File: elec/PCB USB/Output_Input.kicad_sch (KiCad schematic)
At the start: 8 parts, among them J501 Conn_I2C_Écran, SW501 RotaryEncoder_Switch

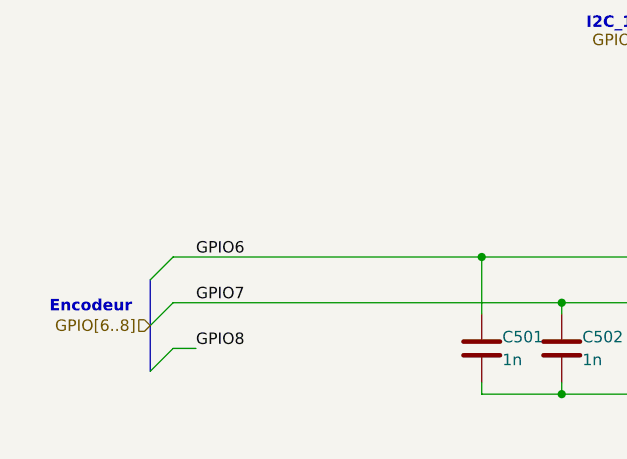
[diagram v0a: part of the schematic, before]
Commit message: push???
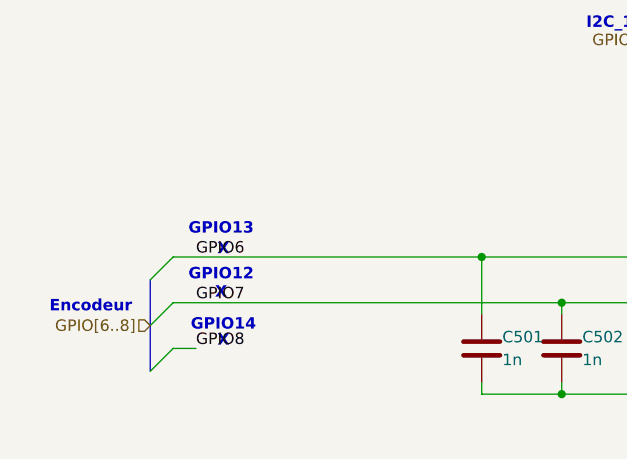
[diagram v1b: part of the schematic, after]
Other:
- note added: "GPIO12"
- note added: "GPIO13"
- note added: "GPIO14"
- note added: "X"
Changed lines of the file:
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@@
+		)
+	)
+	(text "X"
+		(exclude_from_sim no)
+		(at 94.488 84.328 0)
+		(effects
+			(font
+				(size 1.27 1.27)
+				(thickness 0.254)
+				(bold yes)
+				(color 255 24 7 1)
+			)
+		)
+	)
+	(text "GPIO13"
+		(exclude_from_sim no)
+		(at 94.234 71.882 0)
+		(effects
+			(font
+				(size 1.27 1.27)
+				(thickness 0.254)
+				(bold yes)
+				(color 34 86 25 1)
+			)
+		)
+	)
+	(text "X"
+		(exclude_from_sim no)
+		(at 94.488 74.168 0)
+		(effects
+			(font
+				(size 1.27 1.27)
+				(thickness 0.254)
+				(bold yes)
+				(color 255 24 7 1)
+			)
+		)
+	)
+	(text "GPIO14"
+		(exclude_from_sim no)
+		(at 94.488 82.55 0)
+		(effects
+			(font
+				(size 1.27 1.27)
+				(thickness 0.254)
+				(bold yes)
+				(color 34 86 25 1)
+			)
+		)
+	)
+	(text "GPIO12"
+		(exclude_from_sim no)
+		(at 94.234 76.962 0)
+		(effects
+			(font
+				(size 1.27 1.27)
+				(thickness 0.254)
+				(bold yes)
+				(color 34 86 25 1)
+			)
 		)
 	)
@@
 			)
 		)
+	)
+	(text "X"
+		(exclude_from_sim no)
+		(at 94.234 78.994 0)
+		(effects
+			(font
+				(size 1.27 1.27)
+				(thickness 0.254)
+				(bold yes)
+				(color 255 24 7 1)
+			)
+		)
